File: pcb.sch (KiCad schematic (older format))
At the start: 24 parts, among them SW1 SW_Push, U1 ATmega32U4-AU, Y1 Crystal_GND24_Small

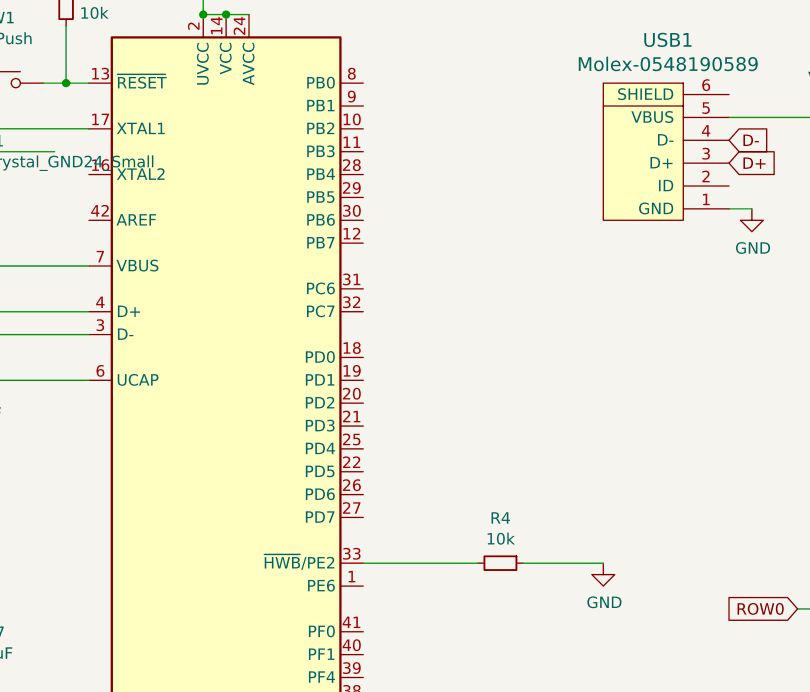
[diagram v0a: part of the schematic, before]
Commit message: yep
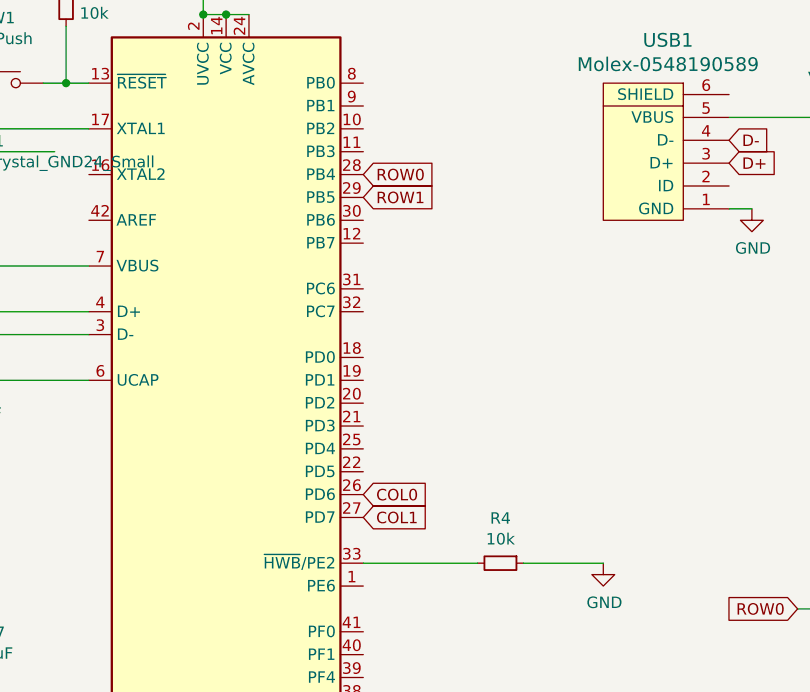
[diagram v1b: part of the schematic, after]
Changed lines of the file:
@@
 Wire Wire Line
 	4750 3050 4550 3050
+Text GLabel 6450 4550 2    50   Input ~ 0
+COL0
+Text GLabel 6450 4650 2    50   Input ~ 0
+COL1
+Text GLabel 6450 3150 2    50   Input ~ 0
+ROW0
+Text GLabel 6450 3250 2    50   Input ~ 0
+ROW1
 $EndSCHEMATC

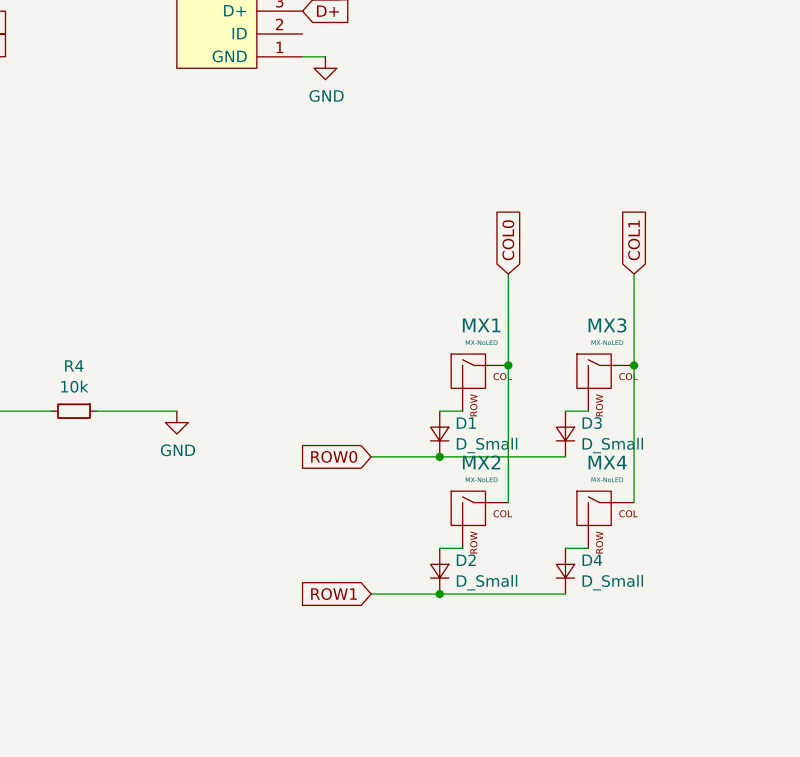
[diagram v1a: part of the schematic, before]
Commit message: add submodules
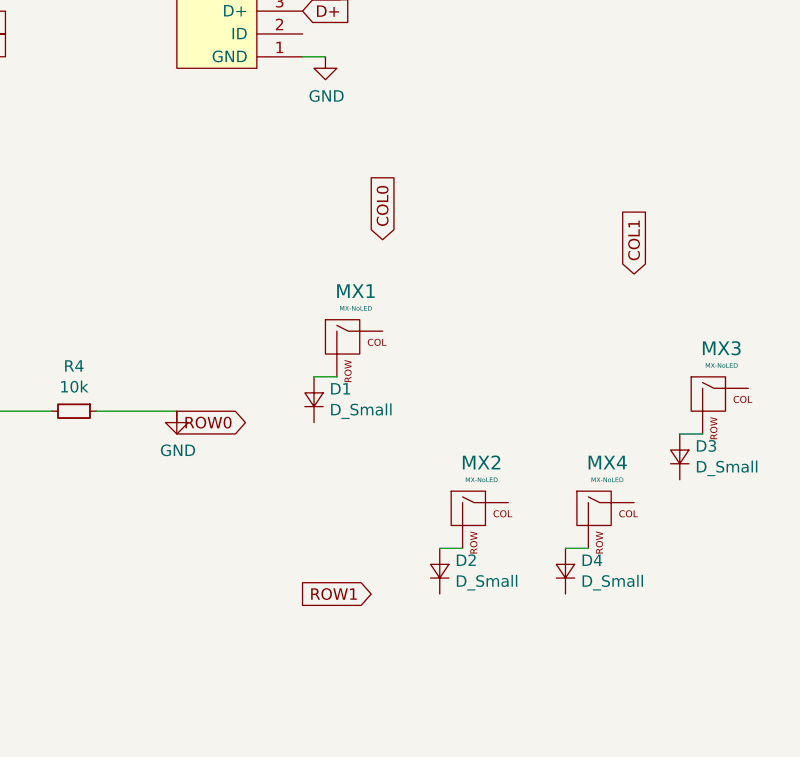
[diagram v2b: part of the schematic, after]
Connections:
- wire segments 61 -> 53
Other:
- moved on the sheet: D1, D3, MX1, MX3
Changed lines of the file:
@@
 L MX_Alps_Hybrid:MX-NoLED MX1
 U 1 1 6315D47E
-P 8800 4700
-F 0 "MX1" H 8833 4923 60  0000 C CNN
-F 1 "MX-NoLED" H 8833 4849 20  0000 C CNN
-F 2 "MX_Alps_Hybrid:MX-1U" H 8175 4675 60  0001 C CNN
-F 3 "" H 8175 4675 60  0001 C CNN
-	1    8800 4700
+P 8250 4550
+F 0 "MX1" H 8283 4773 60  0000 C CNN
+F 1 "MX-NoLED" H 8283 4699 20  0000 C CNN
+F 2 "MX_Alps_Hybrid:MX-1U" H 7625 4525 60  0001 C CNN
+F 3 "" H 7625 4525 60  0001 C CNN
+	1    8250 4550
 	1    0    0    -1
 $EndComp
 Wire Wire Line
-	8750 4850 8650 4850
+	8200 4700 8100 4700
 $Comp
 L Device:D_Small D1
 U 1 1 6315ECF9
-P 8650 4950
-F 0 "D1" V 8696 4882 50  0000 R CNN
-F 1 "D_Small" V 8605 4882 50  0000 R CNN
-F 2 "Diode_SMD:D_SOD-123" V 8650 4950 50  0001 C CNN
-F 3 "~" V 8650 4950 50  0001 C CNN
-	1    8650 4950
+P 8100 4800
+F 0 "D1" V 8146 4732 50  0000 R CNN
+F 1 "D_Small" V 8055 4732 50  0000 R CNN
+F 2 "Diode_SMD:D_SOD-123" V 8100 4800 50  0001 C CNN
+F 3 "~" V 8100 4800 50  0001 C CNN
+	1    8100 4800
 	0    -1   -1   0
 $EndComp
@@
 L MX_Alps_Hybrid:MX-NoLED MX3
 U 1 1 63161B04
-P 9350 4700
-F 0 "MX3" H 9383 4923 60  0000 C CNN
-F 1 "MX-NoLED" H 9383 4849 20  0000 C CNN
-F 2 "MX_Alps_Hybrid:MX-1U" H 8725 4675 60  0001 C CNN
-F 3 "" H 8725 4675 60  0001 C CNN
-	1    9350 4700
+P 9850 4800
+F 0 "MX3" H 9883 5023 60  0000 C CNN
+F 1 "MX-NoLED" H 9883 4949 20  0000 C CNN
+F 2 "MX_Alps_Hybrid:MX-1U" H 9225 4775 60  0001 C CNN
+F 3 "" H 9225 4775 60  0001 C CNN
+	1    9850 4800
 	1    0    0    -1
 $EndComp
@@
 L Device:D_Small D3
 U 1 1 63163246
-P 9200 4950
-F 0 "D3" V 9246 4882 50  0000 R CNN
-F 1 "D_Small" V 9155 4882 50  0000 R CNN
-F 2 "Diode_SMD:D_SOD-123" V 9200 4950 50  0001 C CNN
-F 3 "~" V 9200 4950 50  0001 C CNN
-	1    9200 4950
+P 9700 5050
+F 0 "D3" V 9746 4982 50  0000 R CNN
+F 1 "D_Small" V 9655 4982 50  0000 R CNN
+F 2 "Diode_SMD:D_SOD-123" V 9700 5050 50  0001 C CNN
+F 3 "~" V 9700 5050 50  0001 C CNN
+	1    9700 5050
 	0    -1   -1   0
 $EndComp
 Wire Wire Line
-	9300 4850 9200 4850
+	9800 4950 9700 4950
 $Comp
 L MX_Alps_Hybrid:MX-NoLED MX2
@@
 Wire Wire Line
 	9300 5450 9200 5450
-Wire Wire Line
-	8950 4250 8950 4650
-Connection ~ 8950 4650
-Wire Wire Line
-	8950 4650 8950 5250
-Wire Wire Line
-	9500 4250 9500 4650
-Connection ~ 9500 4650
-Wire Wire Line
-	9500 4650 9500 5250
-Wire Wire Line
-	9200 5650 8650 5650
-Connection ~ 8650 5650
-Wire Wire Line
-	8650 5650 8350 5650
-Wire Wire Line
-	9200 5050 8650 5050
-Connection ~ 8650 5050
-Wire Wire Line
-	8650 5050 8350 5050
-Text GLabel 8350 5050 0    50   Input ~ 0
+Text GLabel 7800 4900 0    50   Input ~ 0
 ROW0
 Text GLabel 8350 5650 0    50   Input ~ 0
 ROW1
-Text GLabel 8950 4250 1    50   Input ~ 0
+Text GLabel 8400 4100 1    50   Input ~ 0
 COL0
 Text GLabel 9500 4250 1    50   Input ~ 0
